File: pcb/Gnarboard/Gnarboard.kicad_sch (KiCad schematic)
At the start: 7 parts, among them U2 MCP3208, U4 D24V5F3

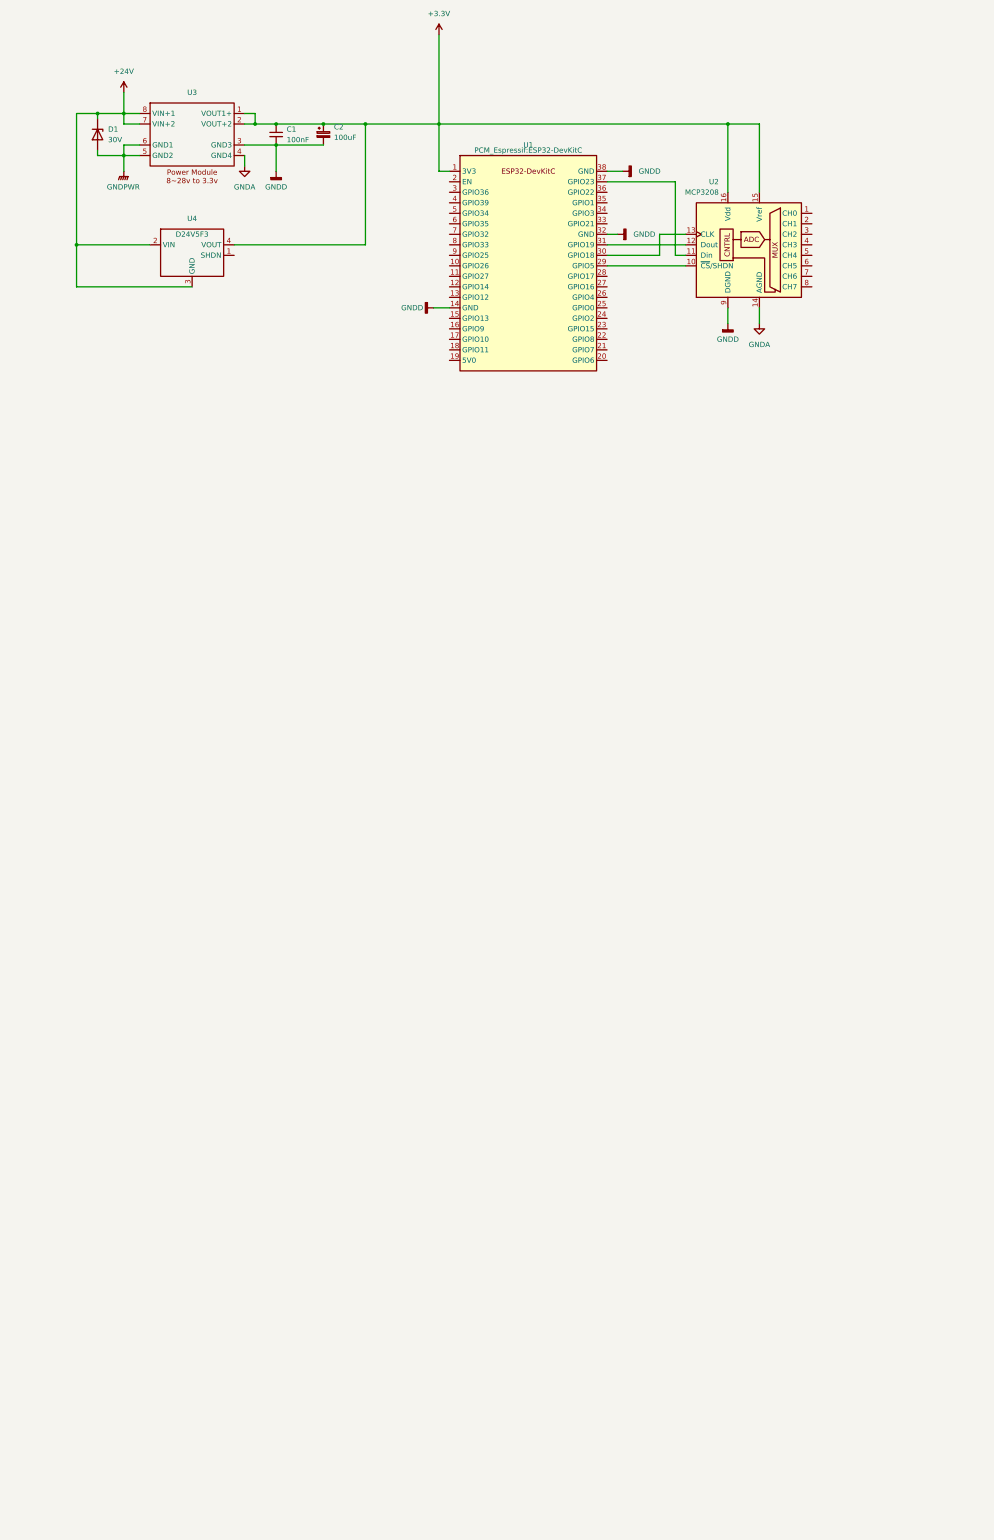
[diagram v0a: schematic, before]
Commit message: much progresso en schematico
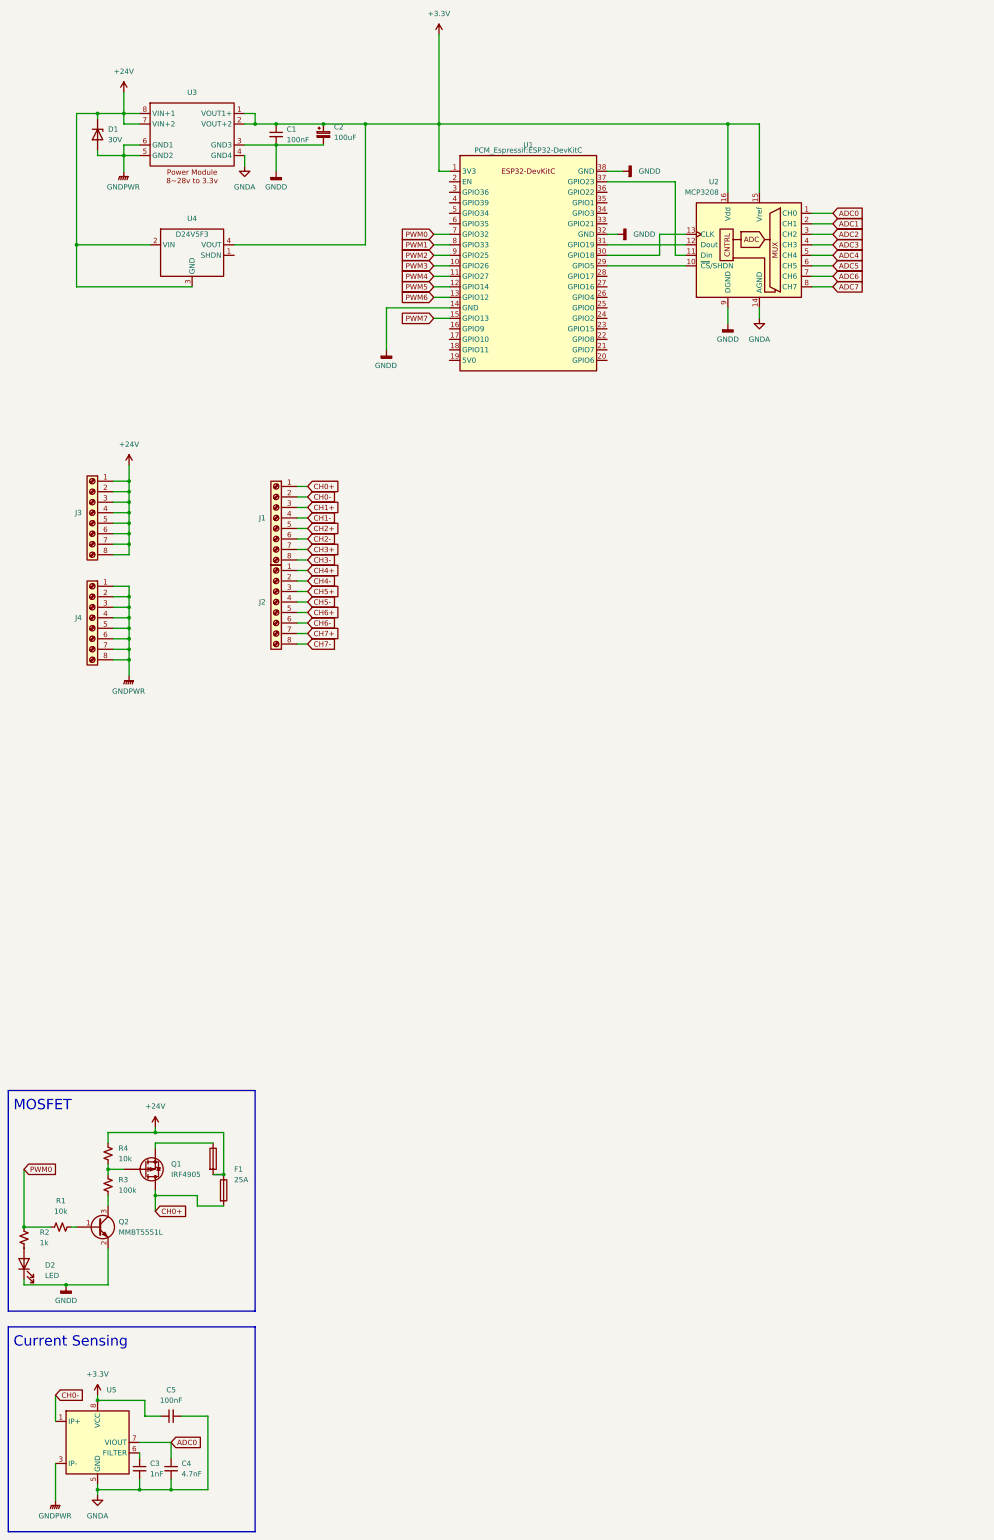
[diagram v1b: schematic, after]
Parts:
- added C3: 1nF, Capacitor_SMD:C_0805_2012Metric_Pad1.18x1.45mm_HandSolder, symbol Device:C_Small
- added C4: 4.7nF, Capacitor_SMD:C_0805_2012Metric_Pad1.18x1.45mm_HandSolder, symbol Device:C_Small
- added C5: 100nF, Capacitor_SMD:C_0805_2012Metric_Pad1.18x1.45mm_HandSolder, symbol Device:C_Small
- added D2: LED, LED_SMD:LED_0805_2012Metric_Pad1.15x1.40mm_HandSolder, symbol Device:LED
- added F1: 25A, gnarboard:ATC Bypass Fuse, symbol gnarboard:ATC Fuse Bypass
- added J1, J2, J3, J4: Screw_Terminal_01x08, Connector_Phoenix_GMSTB:PhoenixContact_GMSTBVA_2,5_8-G_1x08_P7.50mm_Vertical, symbol Connector:Screw_Terminal_01x08
- added Q1: IRF4905, Package_TO_SOT_SMD:TO-263-2, symbol Transistor_FET:IRF4905
- added Q2: MMBT5551L, Package_TO_SOT_SMD:SOT-23, symbol Transistor_BJT:MMBT5551L
- added R1, R4: 10k, Resistor_SMD:R_0805_2012Metric_Pad1.20x1.40mm_HandSolder, symbol Device:R_Small_US
- added R2: 1k, Resistor_SMD:R_0805_2012Metric_Pad1.20x1.40mm_HandSolder, symbol Device:R_Small_US
- added R3: 100k, Resistor_SMD:R_0805_2012Metric_Pad1.20x1.40mm_HandSolder, symbol Device:R_Small_US
- added U5: ACS725xLCTR-20AU, Package_SO:SOIC-8_3.9x4.9mm_P1.27mm, symbol Sensor_Current:ACS725xLCTR-20AU
- C1: footprint Capacitor_THT:C_Disc_D4.7mm_W2.5mm_P5.00mm -> Capacitor_SMD:C_0805_2012Metric_Pad1.18x1.45mm_HandSolder
- U2: footprint Package_DIP:DIP-16_W7.62mm -> Package_SO:SOIC-16_3.9x9.9mm_P1.27mm
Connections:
- net +24V: now also F1.2, J3.1 (Pin_1), J3.2 (Pin_2), J3.3 (Pin_3), J3.4 (Pin_4), J3.5 (Pin_5), J3.6 (Pin_6), J3.7 (Pin_7), J3.8 (Pin_8), R4.2
- net +3.3V: now also C5.1, U5.8 (VCC)
- net GNDA: now also C3.2, C4.2, C5.2, U5.5 (GND)
- net GNDD: now also D2.1 (K), Q2.2 (E)
- net GNDPWR: now also J4.1 (Pin_1), J4.2 (Pin_2), J4.3 (Pin_3), J4.4 (Pin_4), J4.5 (Pin_5), J4.6 (Pin_6), J4.7 (Pin_7), J4.8 (Pin_8), U5.3 (IP-), U5.4 (IP-)
- net ADC0: now reaches U2.1 (CH0)
- net ADC0: now also C4.1, U5.7 (VIOUT)
- net ADC1: now reaches U2.2 (CH1)
- net ADC2: now reaches U2.3 (CH2)
- net ADC3: now reaches U2.4 (CH3)
- net ADC4: now reaches U2.5 (CH4)
- net ADC5: now reaches U2.6 (CH5)
- net ADC6: now reaches U2.7 (CH6)
- net ADC7: now reaches U2.8 (CH7)
- net PWM3: now reaches U1.10 (GPIO26)
- net PWM4: now reaches U1.11 (GPIO27)
- net PWM5: now reaches U1.12 (GPIO14)
- net PWM6: now reaches U1.13 (GPIO12)
- net PWM7: now reaches U1.15 (GPIO13)
- net PWM0: now reaches U1.7 (GPIO32)
- net PWM0: now also R1.1, R2.2
- net PWM1: now reaches U1.8 (GPIO33)
- net PWM2: now reaches U1.9 (GPIO25)
- new net: Q2.1 (B), R1.2
- new net: Q2.3 (C), R3.1
- new net: F1.1, Q1.3 (S)
- new net: C3.1, U5.6 (FILTER)
- new net: D2.2 (A), R2.1
- new net: Q1.1 (G), R3.2, R4.1
- new net CH0+: F1.3, J1.1 (Pin_1), Q1.2 (D)
- new net CH0-: J1.2 (Pin_2), U5.1 (IP+), U5.2 (IP+)
- new net CH1+: J1.3 (Pin_3)
- new net CH1-: J1.4 (Pin_4)
- new net CH2+: J1.5 (Pin_5)
- new net CH2-: J1.6 (Pin_6)
- new net CH3+: J1.7 (Pin_7)
- new net CH3-: J1.8 (Pin_8)
- new net CH4+: J2.1 (Pin_1)
- new net CH4-: J2.2 (Pin_2)
- new net CH5+: J2.3 (Pin_3)
- new net CH5-: J2.4 (Pin_4)
- new net CH6+: J2.5 (Pin_5)
- new net CH6-: J2.6 (Pin_6)
- new net CH7+: J2.7 (Pin_7)
- new net CH7-: J2.8 (Pin_8)
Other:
- note added: "Current Sensing"
- note added: "MOSFET"

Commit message: wow, kicad hierarchical sheets... epic.
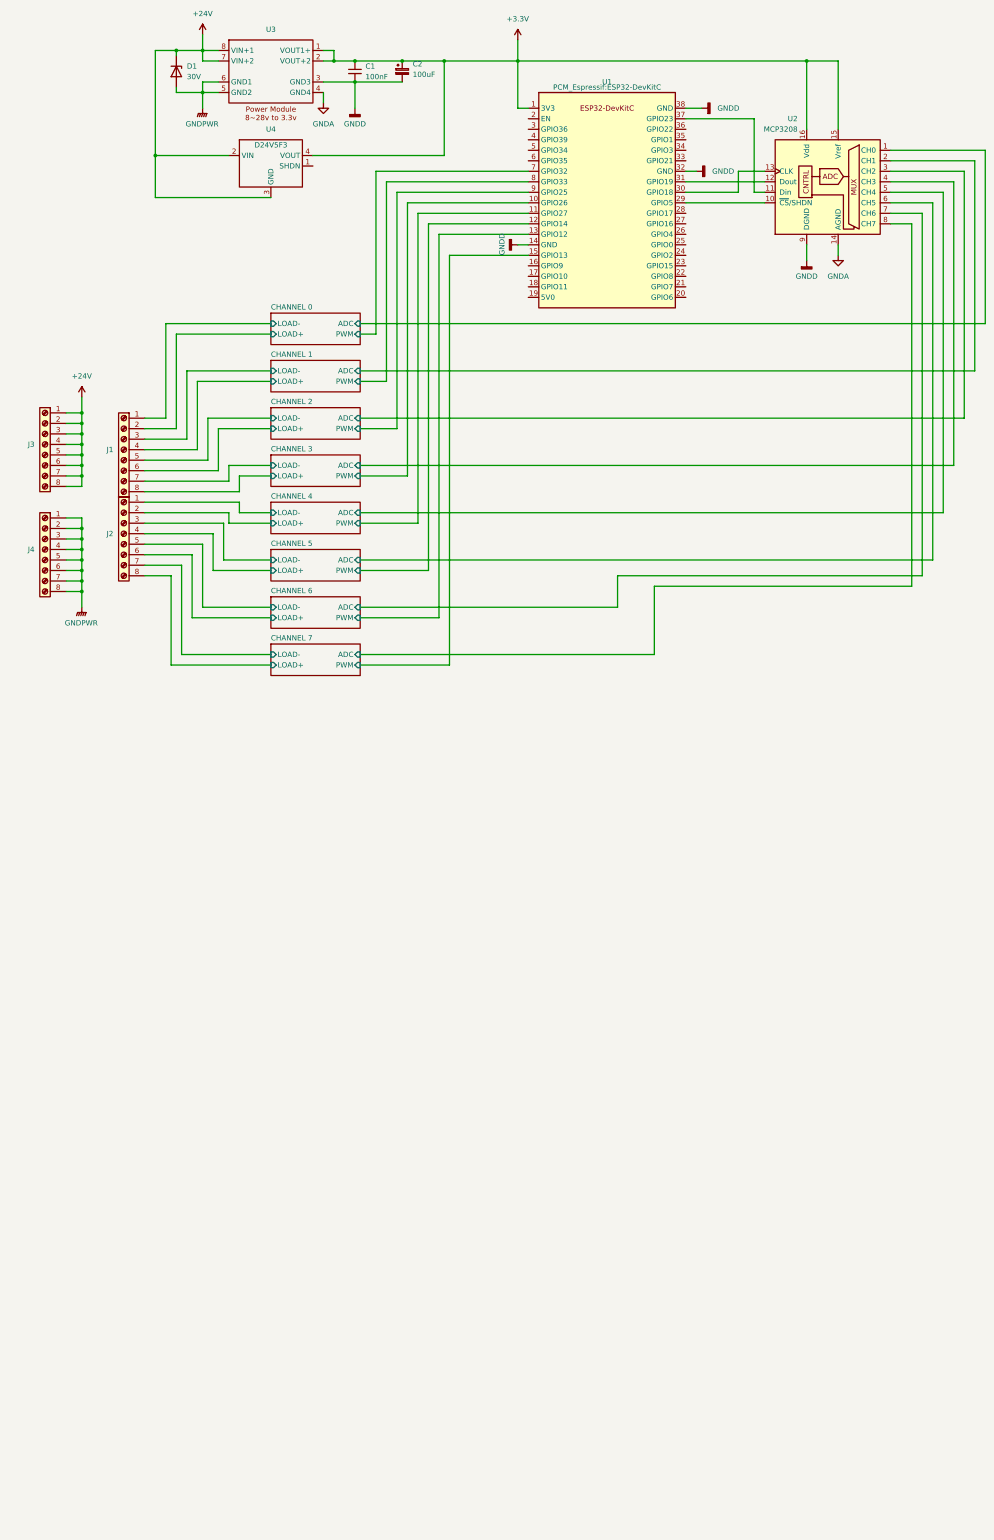
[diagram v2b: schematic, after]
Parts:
- removed C3: 1nF, Capacitor_SMD:C_0805_2012Metric_Pad1.18x1.45mm_HandSolder, symbol Device:C_Small
- removed C4: 4.7nF, Capacitor_SMD:C_0805_2012Metric_Pad1.18x1.45mm_HandSolder, symbol Device:C_Small
- removed C5: 100nF, Capacitor_SMD:C_0805_2012Metric_Pad1.18x1.45mm_HandSolder, symbol Device:C_Small
- removed D2: LED, LED_SMD:LED_0805_2012Metric_Pad1.15x1.40mm_HandSolder, symbol Device:LED
- removed F1: 25A, gnarboard:ATC Bypass Fuse, symbol gnarboard:ATC Fuse Bypass
- removed Q1: IRF4905, Package_TO_SOT_SMD:TO-263-2, symbol Transistor_FET:IRF4905
- removed Q2: MMBT5551L, Package_TO_SOT_SMD:SOT-23, symbol Transistor_BJT:MMBT5551L
- removed R1, R4: 10k, Resistor_SMD:R_0805_2012Metric_Pad1.20x1.40mm_HandSolder, symbol Device:R_Small_US
- removed R2: 1k, Resistor_SMD:R_0805_2012Metric_Pad1.20x1.40mm_HandSolder, symbol Device:R_Small_US
- removed R3: 100k, Resistor_SMD:R_0805_2012Metric_Pad1.20x1.40mm_HandSolder, symbol Device:R_Small_US
- removed U5: ACS725xLCTR-20AU, Package_SO:SOIC-8_3.9x4.9mm_P1.27mm, symbol Sensor_Current:ACS725xLCTR-20AU
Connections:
- net ADC0 renamed CHANNEL 0/ADC
- net ADC1 renamed CHANNEL 1/ADC
- net ADC2 renamed CHANNEL 2/ADC
- net ADC3 renamed CHANNEL 3/ADC
- net ADC4 renamed CHANNEL 4/ADC
- net ADC5 renamed CHANNEL 5/ADC
- net ADC6 renamed CHANNEL 6/ADC
- net ADC7 renamed CHANNEL 7/ADC
- net CH0+ renamed CHANNEL 0/LOAD-
- net CH0- renamed CHANNEL 0/LOAD+
- net CH1+ renamed CHANNEL 1/LOAD-
- net CH1- renamed CHANNEL 1/LOAD+
- net CH2+ renamed CHANNEL 2/LOAD-
- net CH2- renamed CHANNEL 2/LOAD+
- net CH3+ renamed CHANNEL 3/LOAD-
- net CH3- renamed CHANNEL 3/LOAD+
- net CH4+ renamed CHANNEL 4/LOAD-
- net CH4- renamed CHANNEL 4/LOAD+
- net CH5+ renamed CHANNEL 5/LOAD-
- net CH5- renamed CHANNEL 5/LOAD+
- net CH6+ renamed CHANNEL 6/LOAD-
- net CH6- renamed CHANNEL 6/LOAD+
- net CH7+ renamed CHANNEL 7/LOAD-
- net CH7- renamed CHANNEL 7/LOAD+
- net PWM0 renamed CHANNEL 0/PWM
- net PWM1 renamed CHANNEL 1/PWM
- net PWM2 renamed CHANNEL 2/PWM
- net PWM3 renamed CHANNEL 3/PWM
- net PWM4 renamed CHANNEL 4/PWM
- net PWM5 renamed CHANNEL 5/PWM
- net PWM6 renamed CHANNEL 6/PWM
- net PWM7 renamed CHANNEL 7/PWM
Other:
- added sheet CHANNEL 0 (mosfet.kicad_sch)
- added sheet CHANNEL 1 (mosfet.kicad_sch)
- added sheet CHANNEL 2 (mosfet.kicad_sch)
- added sheet CHANNEL 3 (mosfet.kicad_sch)
- added sheet CHANNEL 4 (mosfet.kicad_sch)
- added sheet CHANNEL 5 (mosfet.kicad_sch)
- added sheet CHANNEL 6 (mosfet.kicad_sch)
- added sheet CHANNEL 7 (mosfet.kicad_sch)
- note removed: "Current Sensing"
- note removed: "MOSFET"
- moved on the sheet: C1, C2, D1, J1, J2, J3, J4, U1, U2, U3, U4
